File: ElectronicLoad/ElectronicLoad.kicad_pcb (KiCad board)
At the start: 4 copper layers, 101 x 64 mm, 581 parts, among them J1 AdafruitConverter, J3 Conn_01x02_Female, J4 Conn_01x02_Female, J5 Conn_01x02_Female, Q1 BUK9515-60E, Q2 BUK9515-60E, SW1 Rotary_Encoder_Switch, U1 MCP1812AT-033, U2 STM32G030C6T6, U3 MCP48CXBX1, U4 AD8605, U5 AD8605, U6 AD8605, U7 74HC595D, Y1 Crystal_GND24

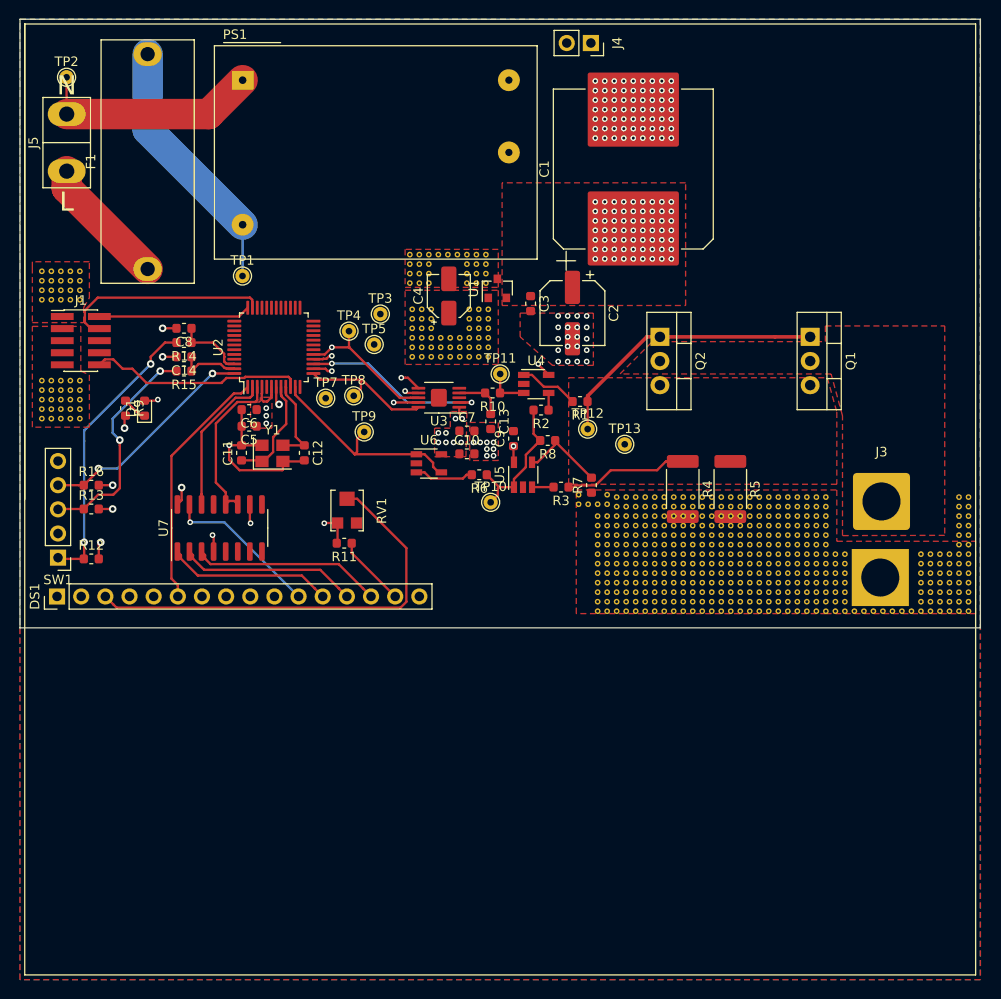
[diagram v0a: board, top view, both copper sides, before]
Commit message: Desktop
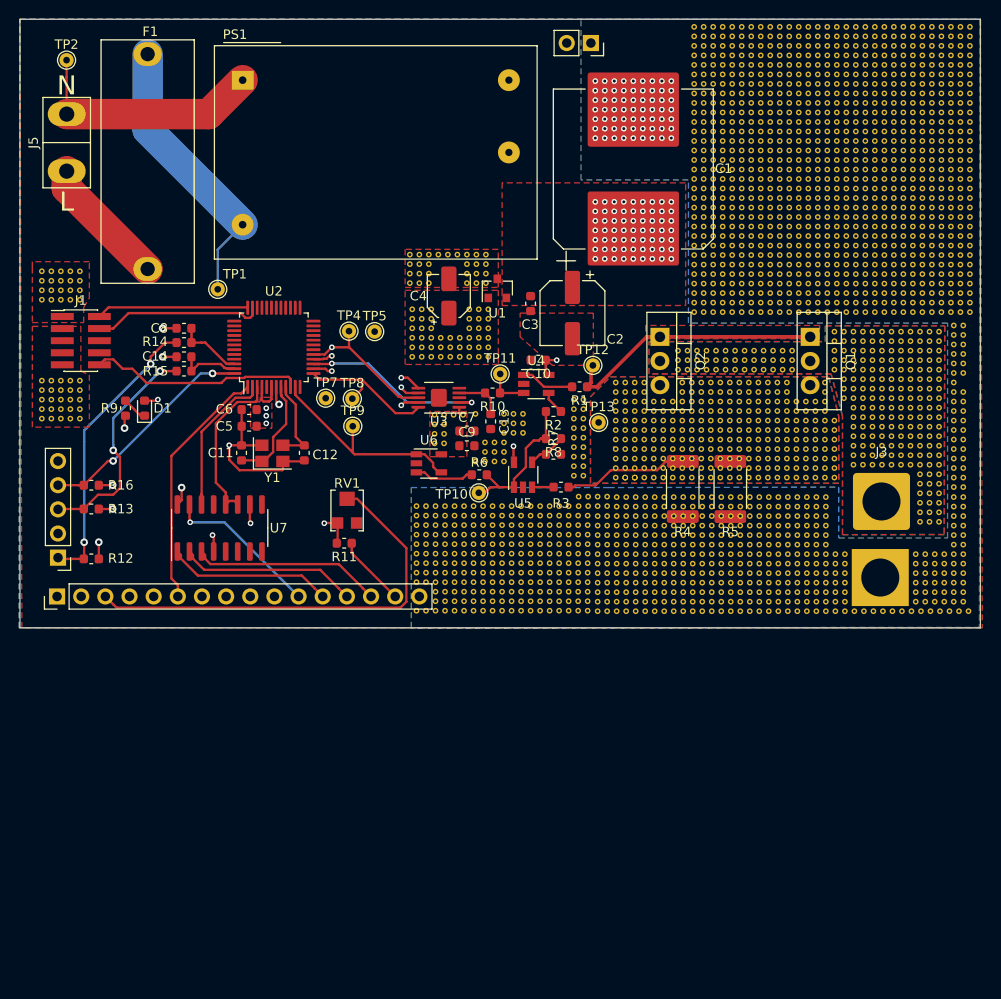
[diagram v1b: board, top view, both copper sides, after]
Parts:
- removed TP3: TestPoint, TestPoint:TestPoint_THTPad_D1.5mm_Drill0.7mm
- added REF**: VIA-0.6mm, Logan:VIA-0.6mm, F.Cu at (64.2, 92.7)
- added REF**: VIA-0.6mm, Logan:VIA-0.6mm, F.Cu at (73.8, 87.5)
- added REF**: VIA-0.6mm, Logan:VIA-0.6mm, F.Cu at (102.4, 72.3)
- added REF**: VIA-0.6mm, Logan:VIA-0.6mm, F.Cu at (102.4, 71.3)
- added REF**: VIA-0.6mm, Logan:VIA-0.6mm, F.Cu at (101.4, 71.3)
- added REF**: VIA-0.6mm, Logan:VIA-0.6mm, F.Cu at (100.4, 71.3)
- added REF**: VIA-0.6mm, Logan:VIA-0.6mm, F.Cu at (99.4, 71.3)
- added REF**: VIA-0.6mm, Logan:VIA-0.6mm, F.Cu at (98.4, 71.3)
- added REF**: VIA-0.6mm, Logan:VIA-0.6mm, F.Cu at (97.4, 71.3)
- added REF**: VIA-0.6mm, Logan:VIA-0.6mm, F.Cu at (96.4, 71.3)
- added REF**: VIA-0.6mm, Logan:VIA-0.6mm, F.Cu at (95.4, 71.3)
- added REF**: VIA-0.6mm, Logan:VIA-0.6mm, F.Cu at (94.4, 71.3)
- added REF**: VIA-0.6mm, Logan:VIA-0.6mm, F.Cu at (93.4, 71.3)
- added REF**: VIA-0.6mm, Logan:VIA-0.6mm, F.Cu at (101.4, 72.3)
- added REF**: VIA-0.6mm, Logan:VIA-0.6mm, F.Cu at (92.4, 71.3)
- added REF**: VIA-0.6mm, Logan:VIA-0.6mm, F.Cu at (91.4, 71.3)
- added REF**: VIA-0.6mm, Logan:VIA-0.6mm, F.Cu at (90.4, 71.3)
- added REF**: VIA-0.6mm, Logan:VIA-0.6mm, F.Cu at (89.4, 71.3)
- added REF**: VIA-0.6mm, Logan:VIA-0.6mm, F.Cu at (88.4, 71.3)
- added REF**: VIA-0.6mm, Logan:VIA-0.6mm, F.Cu at (87.4, 71.3)
- added REF**: VIA-0.6mm, Logan:VIA-0.6mm, F.Cu at (86.4, 71.3)
- added REF**: VIA-0.6mm, Logan:VIA-0.6mm, F.Cu at (101.2, 83.7)
- added REF**: VIA-0.6mm, Logan:VIA-0.6mm, F.Cu at (101.2, 84.7)
- added REF**: VIA-0.6mm, Logan:VIA-0.6mm, F.Cu at (101.2, 85.7)
- added REF**: VIA-0.6mm, Logan:VIA-0.6mm, F.Cu at (100.4, 72.3)
- added REF**: VIA-0.6mm, Logan:VIA-0.6mm, F.Cu at (101.2, 86.7)
- added REF**: VIA-0.6mm, Logan:VIA-0.6mm, F.Cu at (101.2, 87.7)
- added REF**: VIA-0.6mm, Logan:VIA-0.6mm, F.Cu at (101.2, 88.7)
- added REF**: VIA-0.6mm, Logan:VIA-0.6mm, F.Cu at (101.2, 89.7)
- added REF**: VIA-0.6mm, Logan:VIA-0.6mm, F.Cu at (100.2, 89.7)
- added REF**: VIA-0.6mm, Logan:VIA-0.6mm, F.Cu at (99.2, 89.7)
- added REF**: VIA-0.6mm, Logan:VIA-0.6mm, F.Cu at (98.2, 89.7)
- added REF**: VIA-0.6mm, Logan:VIA-0.6mm, F.Cu at (97.2, 89.7)
- added REF**: VIA-0.6mm, Logan:VIA-0.6mm, F.Cu at (96.2, 89.7)
- added REF**: VIA-0.6mm, Logan:VIA-0.6mm, F.Cu at (95.2, 89.7)
- added REF**: VIA-0.6mm, Logan:VIA-0.6mm, F.Cu at (99.4, 72.3)
- added REF**: VIA-0.6mm, Logan:VIA-0.6mm, F.Cu at (94.2, 89.7)
- added REF**: VIA-0.6mm, Logan:VIA-0.6mm, F.Cu at (93.2, 89.7)
- added REF**: VIA-0.6mm, Logan:VIA-0.6mm, F.Cu at (92.2, 89.7)
- added REF**: VIA-0.6mm, Logan:VIA-0.6mm, F.Cu at (91.2, 89.7)
- added REF**: VIA-0.6mm, Logan:VIA-0.6mm, F.Cu at (90.2, 89.7)
- added REF**: VIA-0.6mm, Logan:VIA-0.6mm, F.Cu at (89.2, 89.7)
- added REF**: VIA-0.6mm, Logan:VIA-0.6mm, F.Cu at (88.2, 89.7)
- added REF**: VIA-0.6mm, Logan:VIA-0.6mm, F.Cu at (87.2, 89.7)
- added REF**: VIA-0.6mm, Logan:VIA-0.6mm, F.Cu at (86.2, 89.7)
- added REF**: VIA-0.6mm, Logan:VIA-0.6mm, F.Cu at (85.2, 89.7)
- added REF**: VIA-0.6mm, Logan:VIA-0.6mm, F.Cu at (98.4, 72.3)
- added REF**: VIA-0.6mm, Logan:VIA-0.6mm, F.Cu at (84.2, 89.7)
- added REF**: VIA-0.6mm, Logan:VIA-0.6mm, F.Cu at (83.2, 89.7)
- added REF**: VIA-0.6mm, Logan:VIA-0.6mm, F.Cu at (82.2, 89.7)
- added REF**: VIA-0.6mm, Logan:VIA-0.6mm, F.Cu at (81.2, 89.7)
- added REF** (x2): VIA-0.6mm, Logan:VIA-0.6mm, F.Cu at (80.2, 89.7)
- added REF** (x2): VIA-0.6mm, Logan:VIA-0.6mm, F.Cu at (79.2, 89.7)
- added REF**: VIA-0.6mm, Logan:VIA-0.6mm, F.Cu at (100.2, 88.7)
- added REF**: VIA-0.6mm, Logan:VIA-0.6mm, F.Cu at (99.2, 88.7)
- added REF**: VIA-0.6mm, Logan:VIA-0.6mm, F.Cu at (98.2, 88.7)
- added REF**: VIA-0.6mm, Logan:VIA-0.6mm, F.Cu at (97.2, 88.7)
- added REF**: VIA-0.6mm, Logan:VIA-0.6mm, F.Cu at (97.4, 72.3)
- added REF**: VIA-0.6mm, Logan:VIA-0.6mm, F.Cu at (96.2, 88.7)
- added REF**: VIA-0.6mm, Logan:VIA-0.6mm, F.Cu at (95.2, 88.7)
- added REF**: VIA-0.6mm, Logan:VIA-0.6mm, F.Cu at (94.2, 88.7)
- added REF**: VIA-0.6mm, Logan:VIA-0.6mm, F.Cu at (93.2, 88.7)
- added REF**: VIA-0.6mm, Logan:VIA-0.6mm, F.Cu at (92.2, 88.7)
- added REF**: VIA-0.6mm, Logan:VIA-0.6mm, F.Cu at (91.2, 88.7)
- added REF**: VIA-0.6mm, Logan:VIA-0.6mm, F.Cu at (90.2, 88.7)
- added REF**: VIA-0.6mm, Logan:VIA-0.6mm, F.Cu at (89.2, 88.7)
- added REF**: VIA-0.6mm, Logan:VIA-0.6mm, F.Cu at (88.2, 88.7)
- added REF**: VIA-0.6mm, Logan:VIA-0.6mm, F.Cu at (87.2, 88.7)
- added REF**: VIA-0.6mm, Logan:VIA-0.6mm, F.Cu at (96.4, 72.3)
- added REF**: VIA-0.6mm, Logan:VIA-0.6mm, F.Cu at (86.2, 88.7)
- added REF**: VIA-0.6mm, Logan:VIA-0.6mm, F.Cu at (85.2, 88.7)
- added REF**: VIA-0.6mm, Logan:VIA-0.6mm, F.Cu at (84.2, 88.7)
- added REF**: VIA-0.6mm, Logan:VIA-0.6mm, F.Cu at (83.2, 88.7)
- added REF**: VIA-0.6mm, Logan:VIA-0.6mm, F.Cu at (82.2, 88.7)
- added REF**: VIA-0.6mm, Logan:VIA-0.6mm, F.Cu at (81.2, 88.7)
- added REF**: VIA-0.6mm, Logan:VIA-0.6mm, F.Cu at (100.2, 87.7)
- added REF**: VIA-0.6mm, Logan:VIA-0.6mm, F.Cu at (99.2, 87.7)
- added REF**: VIA-0.6mm, Logan:VIA-0.6mm, F.Cu at (98.2, 87.7)
- added REF**: VIA-0.6mm, Logan:VIA-0.6mm, F.Cu at (97.2, 87.7)
- added REF**: VIA-0.6mm, Logan:VIA-0.6mm, F.Cu at (95.4, 72.3)
- added REF**: VIA-0.6mm, Logan:VIA-0.6mm, F.Cu at (96.2, 87.7)
- added REF**: VIA-0.6mm, Logan:VIA-0.6mm, F.Cu at (95.2, 87.7)
- added REF**: VIA-0.6mm, Logan:VIA-0.6mm, F.Cu at (94.2, 87.7)
- added REF**: VIA-0.6mm, Logan:VIA-0.6mm, F.Cu at (93.2, 87.7)
- added REF**: VIA-0.6mm, Logan:VIA-0.6mm, F.Cu at (92.2, 87.7)
- added REF**: VIA-0.6mm, Logan:VIA-0.6mm, F.Cu at (91.2, 87.7)
- added REF**: VIA-0.6mm, Logan:VIA-0.6mm, F.Cu at (90.2, 87.7)
- added REF**: VIA-0.6mm, Logan:VIA-0.6mm, F.Cu at (89.2, 87.7)
- added REF**: VIA-0.6mm, Logan:VIA-0.6mm, F.Cu at (88.2, 87.7)
- added REF**: VIA-0.6mm, Logan:VIA-0.6mm, F.Cu at (87.2, 87.7)
- added REF**: VIA-0.6mm, Logan:VIA-0.6mm, F.Cu at (94.4, 72.3)
- added REF**: VIA-0.6mm, Logan:VIA-0.6mm, F.Cu at (86.2, 87.7)
- added REF**: VIA-0.6mm, Logan:VIA-0.6mm, F.Cu at (85.2, 87.7)
- added REF**: VIA-0.6mm, Logan:VIA-0.6mm, F.Cu at (84.2, 87.7)
- added REF**: VIA-0.6mm, Logan:VIA-0.6mm, F.Cu at (83.2, 87.7)
- added REF**: VIA-0.6mm, Logan:VIA-0.6mm, F.Cu at (82.2, 87.7)
- added REF**: VIA-0.6mm, Logan:VIA-0.6mm, F.Cu at (81.2, 87.7)
- added REF**: VIA-0.6mm, Logan:VIA-0.6mm, F.Cu at (100.2, 86.7)
- added REF**: VIA-0.6mm, Logan:VIA-0.6mm, F.Cu at (99.2, 86.7)
- added REF**: VIA-0.6mm, Logan:VIA-0.6mm, F.Cu at (98.2, 86.7)
- added REF**: VIA-0.6mm, Logan:VIA-0.6mm, F.Cu at (97.2, 86.7)
- added REF**: VIA-0.6mm, Logan:VIA-0.6mm, F.Cu at (93.4, 72.3)
- added REF**: VIA-0.6mm, Logan:VIA-0.6mm, F.Cu at (96.2, 86.7)
- added REF**: VIA-0.6mm, Logan:VIA-0.6mm, F.Cu at (95.2, 86.7)
- added REF**: VIA-0.6mm, Logan:VIA-0.6mm, F.Cu at (94.2, 86.7)
- added REF**: VIA-0.6mm, Logan:VIA-0.6mm, F.Cu at (93.2, 86.7)
- added REF**: VIA-0.6mm, Logan:VIA-0.6mm, F.Cu at (92.2, 86.7)
- added REF**: VIA-0.6mm, Logan:VIA-0.6mm, F.Cu at (91.2, 86.7)
- added REF**: VIA-0.6mm, Logan:VIA-0.6mm, F.Cu at (90.2, 86.7)
- added REF**: VIA-0.6mm, Logan:VIA-0.6mm, F.Cu at (89.2, 86.7)
- added REF**: VIA-0.6mm, Logan:VIA-0.6mm, F.Cu at (88.2, 86.7)
- added REF**: VIA-0.6mm, Logan:VIA-0.6mm, F.Cu at (87.2, 86.7)
- added REF**: VIA-0.6mm, Logan:VIA-0.6mm, F.Cu at (73.8, 88.5)
- added REF**: VIA-0.6mm, Logan:VIA-0.6mm, F.Cu at (92.4, 72.3)
- added REF**: VIA-0.6mm, Logan:VIA-0.6mm, F.Cu at (86.2, 86.7)
- added REF**: VIA-0.6mm, Logan:VIA-0.6mm, F.Cu at (85.2, 86.7)
- added REF**: VIA-0.6mm, Logan:VIA-0.6mm, F.Cu at (84.2, 86.7)
- added REF**: VIA-0.6mm, Logan:VIA-0.6mm, F.Cu at (83.2, 86.7)
- added REF**: VIA-0.6mm, Logan:VIA-0.6mm, F.Cu at (82.2, 86.7)
- added REF**: VIA-0.6mm, Logan:VIA-0.6mm, F.Cu at (81.2, 86.7)
- added REF**: VIA-0.6mm, Logan:VIA-0.6mm, F.Cu at (100.2, 85.7)
- added REF**: VIA-0.6mm, Logan:VIA-0.6mm, F.Cu at (99.2, 85.7)
- added REF**: VIA-0.6mm, Logan:VIA-0.6mm, F.Cu at (98.2, 85.7)
- added REF**: VIA-0.6mm, Logan:VIA-0.6mm, F.Cu at (97.2, 85.7)
- added REF**: VIA-0.6mm, Logan:VIA-0.6mm, F.Cu at (91.4, 72.3)
- added REF**: VIA-0.6mm, Logan:VIA-0.6mm, F.Cu at (96.2, 85.7)
- added REF**: VIA-0.6mm, Logan:VIA-0.6mm, F.Cu at (95.2, 85.7)
- added REF**: VIA-0.6mm, Logan:VIA-0.6mm, F.Cu at (94.2, 85.7)
- added REF**: VIA-0.6mm, Logan:VIA-0.6mm, F.Cu at (93.2, 85.7)
- added REF**: VIA-0.6mm, Logan:VIA-0.6mm, F.Cu at (92.2, 85.7)
- added REF**: VIA-0.6mm, Logan:VIA-0.6mm, F.Cu at (91.2, 85.7)
- added REF**: VIA-0.6mm, Logan:VIA-0.6mm, F.Cu at (90.2, 85.7)
- added REF**: VIA-0.6mm, Logan:VIA-0.6mm, F.Cu at (89.2, 85.7)
- added REF**: VIA-0.6mm, Logan:VIA-0.6mm, F.Cu at (88.2, 85.7)
- added REF**: VIA-0.6mm, Logan:VIA-0.6mm, F.Cu at (87.2, 85.7)
- added REF**: VIA-0.6mm, Logan:VIA-0.6mm, F.Cu at (90.4, 72.3)
- added REF**: VIA-0.6mm, Logan:VIA-0.6mm, F.Cu at (86.2, 85.7)
- added REF**: VIA-0.6mm, Logan:VIA-0.6mm, F.Cu at (85.2, 85.7)
- added REF**: VIA-0.6mm, Logan:VIA-0.6mm, F.Cu at (84.2, 85.7)
- added REF**: VIA-0.6mm, Logan:VIA-0.6mm, F.Cu at (83.2, 85.7)
- added REF**: VIA-0.6mm, Logan:VIA-0.6mm, F.Cu at (82.2, 85.7)
- added REF**: VIA-0.6mm, Logan:VIA-0.6mm, F.Cu at (81.2, 85.7)
- added REF**: VIA-0.6mm, Logan:VIA-0.6mm, F.Cu at (100.2, 84.7)
- added REF**: VIA-0.6mm, Logan:VIA-0.6mm, F.Cu at (99.2, 84.7)
- added REF**: VIA-0.6mm, Logan:VIA-0.6mm, F.Cu at (98.2, 84.7)
- added REF**: VIA-0.6mm, Logan:VIA-0.6mm, F.Cu at (97.2, 84.7)
- added REF**: VIA-0.6mm, Logan:VIA-0.6mm, F.Cu at (89.4, 72.3)
- added REF**: VIA-0.6mm, Logan:VIA-0.6mm, F.Cu at (96.2, 84.7)
- added REF**: VIA-0.6mm, Logan:VIA-0.6mm, F.Cu at (95.2, 84.7)
- added REF**: VIA-0.6mm, Logan:VIA-0.6mm, F.Cu at (94.2, 84.7)
- added REF**: VIA-0.6mm, Logan:VIA-0.6mm, F.Cu at (93.2, 84.7)
- added REF**: VIA-0.6mm, Logan:VIA-0.6mm, F.Cu at (92.2, 84.7)
- added REF**: VIA-0.6mm, Logan:VIA-0.6mm, F.Cu at (91.2, 84.7)
- added REF**: VIA-0.6mm, Logan:VIA-0.6mm, F.Cu at (90.2, 84.7)
- added REF**: VIA-0.6mm, Logan:VIA-0.6mm, F.Cu at (89.2, 84.7)
- added REF**: VIA-0.6mm, Logan:VIA-0.6mm, F.Cu at (88.2, 84.7)
- added REF**: VIA-0.6mm, Logan:VIA-0.6mm, F.Cu at (87.2, 84.7)
- added REF**: VIA-0.6mm, Logan:VIA-0.6mm, F.Cu at (88.4, 72.3)
- added REF**: VIA-0.6mm, Logan:VIA-0.6mm, F.Cu at (86.2, 84.7)
- added REF**: VIA-0.6mm, Logan:VIA-0.6mm, F.Cu at (85.2, 84.7)
- added REF**: VIA-0.6mm, Logan:VIA-0.6mm, F.Cu at (84.2, 84.7)
- added REF**: VIA-0.6mm, Logan:VIA-0.6mm, F.Cu at (83.2, 84.7)
- added REF**: VIA-0.6mm, Logan:VIA-0.6mm, F.Cu at (82.2, 84.7)
- added REF**: VIA-0.6mm, Logan:VIA-0.6mm, F.Cu at (81.2, 84.7)
- added REF**: VIA-0.6mm, Logan:VIA-0.6mm, F.Cu at (78.2, 79.7)
- added REF**: VIA-0.6mm, Logan:VIA-0.6mm, F.Cu at (79.2, 79.7)
- added REF**: VIA-0.6mm, Logan:VIA-0.6mm, F.Cu at (80.2, 79.7)
- added REF**: VIA-0.6mm, Logan:VIA-0.6mm, F.Cu at (100.2, 83.7)
- added REF**: VIA-0.6mm, Logan:VIA-0.6mm, F.Cu at (87.4, 72.3)
- added REF**: VIA-0.6mm, Logan:VIA-0.6mm, F.Cu at (99.2, 83.7)
- added REF**: VIA-0.6mm, Logan:VIA-0.6mm, F.Cu at (98.2, 83.7)
- added REF**: VIA-0.6mm, Logan:VIA-0.6mm, F.Cu at (97.2, 83.7)
- added REF**: VIA-0.6mm, Logan:VIA-0.6mm, F.Cu at (96.2, 83.7)
- added REF**: VIA-0.6mm, Logan:VIA-0.6mm, F.Cu at (95.2, 83.7)
- added REF**: VIA-0.6mm, Logan:VIA-0.6mm, F.Cu at (94.2, 83.7)
- added REF**: VIA-0.6mm, Logan:VIA-0.6mm, F.Cu at (93.2, 83.7)
- added REF**: VIA-0.6mm, Logan:VIA-0.6mm, F.Cu at (92.2, 83.7)
- added REF**: VIA-0.6mm, Logan:VIA-0.6mm, F.Cu at (91.2, 83.7)
- added REF**: VIA-0.6mm, Logan:VIA-0.6mm, F.Cu at (90.2, 83.7)
- added REF**: VIA-0.6mm, Logan:VIA-0.6mm, F.Cu at (86.4, 72.3)
- added REF**: VIA-0.6mm, Logan:VIA-0.6mm, F.Cu at (89.2, 83.7)
- added REF**: VIA-0.6mm, Logan:VIA-0.6mm, F.Cu at (88.2, 83.7)
- added REF**: VIA-0.6mm, Logan:VIA-0.6mm, F.Cu at (87.2, 83.7)
- added REF**: VIA-0.6mm, Logan:VIA-0.6mm, F.Cu at (86.2, 83.7)
- added REF**: VIA-0.6mm, Logan:VIA-0.6mm, F.Cu at (85.2, 83.7)
- added REF**: VIA-0.6mm, Logan:VIA-0.6mm, F.Cu at (84.2, 83.7)
- added REF**: VIA-0.6mm, Logan:VIA-0.6mm, F.Cu at (83.2, 83.7)
- added REF**: VIA-0.6mm, Logan:VIA-0.6mm, F.Cu at (82.2, 83.7)
- added REF**: VIA-0.6mm, Logan:VIA-0.6mm, F.Cu at (81.2, 83.7)
- added REF**: VIA-0.6mm, Logan:VIA-0.6mm, F.Cu at (78.2, 80.7)
- added REF**: VIA-0.6mm, Logan:VIA-0.6mm, F.Cu at (115.4, 42.3)
- added REF**: VIA-0.6mm, Logan:VIA-0.6mm, F.Cu at (79.2, 80.7)
- added REF**: VIA-0.6mm, Logan:VIA-0.6mm, F.Cu at (80.2, 80.7)
- added REF**: VIA-0.6mm, Logan:VIA-0.6mm, F.Cu at (100.2, 82.7)
- added REF**: VIA-0.6mm, Logan:VIA-0.6mm, F.Cu at (99.2, 82.7)
- added REF**: VIA-0.6mm, Logan:VIA-0.6mm, F.Cu at (98.2, 82.7)
- added REF**: VIA-0.6mm, Logan:VIA-0.6mm, F.Cu at (97.2, 82.7)
- added REF**: VIA-0.6mm, Logan:VIA-0.6mm, F.Cu at (96.2, 82.7)
- added REF**: VIA-0.6mm, Logan:VIA-0.6mm, F.Cu at (95.2, 82.7)
- added REF**: VIA-0.6mm, Logan:VIA-0.6mm, F.Cu at (94.2, 82.7)
- added REF**: VIA-0.6mm, Logan:VIA-0.6mm, F.Cu at (93.2, 82.7)
- added REF**: VIA-0.6mm, Logan:VIA-0.6mm, F.Cu at (114.4, 42.3)
- added REF**: VIA-0.6mm, Logan:VIA-0.6mm, F.Cu at (92.2, 82.7)
- added REF**: VIA-0.6mm, Logan:VIA-0.6mm, F.Cu at (91.2, 82.7)
- added REF**: VIA-0.6mm, Logan:VIA-0.6mm, F.Cu at (90.2, 82.7)
- added REF**: VIA-0.6mm, Logan:VIA-0.6mm, F.Cu at (89.2, 82.7)
- added REF**: VIA-0.6mm, Logan:VIA-0.6mm, F.Cu at (88.2, 82.7)
- added REF**: VIA-0.6mm, Logan:VIA-0.6mm, F.Cu at (87.2, 82.7)
- added REF**: VIA-0.6mm, Logan:VIA-0.6mm, F.Cu at (86.2, 82.7)
- added REF**: VIA-0.6mm, Logan:VIA-0.6mm, F.Cu at (85.2, 82.7)
- added REF**: VIA-0.6mm, Logan:VIA-0.6mm, F.Cu at (84.2, 82.7)
- added REF**: VIA-0.6mm, Logan:VIA-0.6mm, F.Cu at (83.2, 82.7)
- added REF**: VIA-0.6mm, Logan:VIA-0.6mm, F.Cu at (113.4, 42.3)
- added REF**: VIA-0.6mm, Logan:VIA-0.6mm, F.Cu at (82.2, 82.7)
- added REF**: VIA-0.6mm, Logan:VIA-0.6mm, F.Cu at (81.2, 82.7)
- added REF**: VIA-0.6mm, Logan:VIA-0.6mm, F.Cu at (78.2, 81.7)
- added REF**: VIA-0.6mm, Logan:VIA-0.6mm, F.Cu at (79.2, 81.7)
- added REF**: VIA-0.6mm, Logan:VIA-0.6mm, F.Cu at (80.2, 81.7)
- added REF**: VIA-0.6mm, Logan:VIA-0.6mm, F.Cu at (100.2, 81.7)
- added REF**: VIA-0.6mm, Logan:VIA-0.6mm, F.Cu at (99.2, 81.7)
- added REF**: VIA-0.6mm, Logan:VIA-0.6mm, F.Cu at (98.2, 81.7)
- added REF**: VIA-0.6mm, Logan:VIA-0.6mm, F.Cu at (97.2, 81.7)
- added REF**: VIA-0.6mm, Logan:VIA-0.6mm, F.Cu at (96.2, 81.7)
- added REF**: VIA-0.6mm, Logan:VIA-0.6mm, F.Cu at (73.8, 89.5)
- added REF**: VIA-0.6mm, Logan:VIA-0.6mm, F.Cu at (112.4, 42.3)
- added REF**: VIA-0.6mm, Logan:VIA-0.6mm, F.Cu at (95.2, 81.7)
- added REF**: VIA-0.6mm, Logan:VIA-0.6mm, F.Cu at (94.2, 81.7)
- added REF**: VIA-0.6mm, Logan:VIA-0.6mm, F.Cu at (93.2, 81.7)
- added REF**: VIA-0.6mm, Logan:VIA-0.6mm, F.Cu at (92.2, 81.7)
- added REF**: VIA-0.6mm, Logan:VIA-0.6mm, F.Cu at (91.2, 81.7)
- added REF**: VIA-0.6mm, Logan:VIA-0.6mm, F.Cu at (90.2, 81.7)
- added REF**: VIA-0.6mm, Logan:VIA-0.6mm, F.Cu at (89.2, 81.7)
- added REF**: VIA-0.6mm, Logan:VIA-0.6mm, F.Cu at (88.2, 81.7)
- added REF**: VIA-0.6mm, Logan:VIA-0.6mm, F.Cu at (87.2, 81.7)
- added REF**: VIA-0.6mm, Logan:VIA-0.6mm, F.Cu at (86.2, 81.7)
- added REF**: VIA-0.6mm, Logan:VIA-0.6mm, F.Cu at (111.4, 42.3)
- added REF**: VIA-0.6mm, Logan:VIA-0.6mm, F.Cu at (85.2, 81.7)
- added REF**: VIA-0.6mm, Logan:VIA-0.6mm, F.Cu at (84.2, 81.7)
- added REF**: VIA-0.6mm, Logan:VIA-0.6mm, F.Cu at (83.2, 81.7)
- added REF**: VIA-0.6mm, Logan:VIA-0.6mm, F.Cu at (82.2, 81.7)
- added REF**: VIA-0.6mm, Logan:VIA-0.6mm, F.Cu at (81.2, 81.7)
- added REF**: VIA-0.6mm, Logan:VIA-0.6mm, F.Cu at (78.2, 82.7)
- added REF**: VIA-0.6mm, Logan:VIA-0.6mm, F.Cu at (79.2, 82.7)
- added REF**: VIA-0.6mm, Logan:VIA-0.6mm, F.Cu at (80.2, 82.7)
- added REF**: VIA-0.6mm, Logan:VIA-0.6mm, F.Cu at (100.2, 80.7)
- added REF**: VIA-0.6mm, Logan:VIA-0.6mm, F.Cu at (96.2, 80.7)
- added REF**: VIA-0.6mm, Logan:VIA-0.6mm, F.Cu at (110.4, 42.3)
- added REF**: VIA-0.6mm, Logan:VIA-0.6mm, F.Cu at (95.2, 80.7)
- added REF**: VIA-0.6mm, Logan:VIA-0.6mm, F.Cu at (94.2, 80.7)
- added REF**: VIA-0.6mm, Logan:VIA-0.6mm, F.Cu at (93.2, 80.7)
- added REF**: VIA-0.6mm, Logan:VIA-0.6mm, F.Cu at (92.2, 80.7)
- added REF**: VIA-0.6mm, Logan:VIA-0.6mm, F.Cu at (91.2, 80.7)
- added REF**: VIA-0.6mm, Logan:VIA-0.6mm, F.Cu at (90.2, 80.7)
- added REF**: VIA-0.6mm, Logan:VIA-0.6mm, F.Cu at (89.2, 80.7)
- added REF**: VIA-0.6mm, Logan:VIA-0.6mm, F.Cu at (88.2, 80.7)
- added REF**: VIA-0.6mm, Logan:VIA-0.6mm, F.Cu at (87.2, 80.7)
- added REF**: VIA-0.6mm, Logan:VIA-0.6mm, F.Cu at (86.2, 80.7)
- added REF**: VIA-0.6mm, Logan:VIA-0.6mm, F.Cu at (109.4, 42.3)
- added REF**: VIA-0.6mm, Logan:VIA-0.6mm, F.Cu at (85.2, 80.7)
- added REF**: VIA-0.6mm, Logan:VIA-0.6mm, F.Cu at (81.2, 80.7)
- added REF**: VIA-0.6mm, Logan:VIA-0.6mm, F.Cu at (78.2, 83.7)
- added REF**: VIA-0.6mm, Logan:VIA-0.6mm, F.Cu at (79.2, 83.7)
- added REF**: VIA-0.6mm, Logan:VIA-0.6mm, F.Cu at (80.2, 83.7)
- added REF**: VIA-0.6mm, Logan:VIA-0.6mm, F.Cu at (100.2, 79.7)
- added REF**: VIA-0.6mm, Logan:VIA-0.6mm, F.Cu at (96.2, 79.7)
- added REF**: VIA-0.6mm, Logan:VIA-0.6mm, F.Cu at (95.2, 79.7)
- added REF**: VIA-0.6mm, Logan:VIA-0.6mm, F.Cu at (94.2, 79.7)
- added REF**: VIA-0.6mm, Logan:VIA-0.6mm, F.Cu at (93.2, 79.7)
- added REF**: VIA-0.6mm, Logan:VIA-0.6mm, F.Cu at (108.4, 42.3)
- added REF**: VIA-0.6mm, Logan:VIA-0.6mm, F.Cu at (92.2, 79.7)
- added REF**: VIA-0.6mm, Logan:VIA-0.6mm, F.Cu at (91.2, 79.7)
- added REF**: VIA-0.6mm, Logan:VIA-0.6mm, F.Cu at (90.2, 79.7)
- added REF**: VIA-0.6mm, Logan:VIA-0.6mm, F.Cu at (89.2, 79.7)
- added REF**: VIA-0.6mm, Logan:VIA-0.6mm, F.Cu at (88.2, 79.7)
- added REF**: VIA-0.6mm, Logan:VIA-0.6mm, F.Cu at (87.2, 79.7)
- added REF**: VIA-0.6mm, Logan:VIA-0.6mm, F.Cu at (86.2, 79.7)
- added REF**: VIA-0.6mm, Logan:VIA-0.6mm, F.Cu at (85.2, 79.7)
- added REF**: VIA-0.6mm, Logan:VIA-0.6mm, F.Cu at (81.2, 79.7)
- added REF**: VIA-0.6mm, Logan:VIA-0.6mm, F.Cu at (78.2, 84.7)
- added REF**: VIA-0.6mm, Logan:VIA-0.6mm, F.Cu at (107.4, 42.3)
- added REF**: VIA-0.6mm, Logan:VIA-0.6mm, F.Cu at (79.2, 84.7)
- added REF**: VIA-0.6mm, Logan:VIA-0.6mm, F.Cu at (80.2, 84.7)
- added REF**: VIA-0.6mm, Logan:VIA-0.6mm, F.Cu at (78.2, 85.7)
- added REF**: VIA-0.6mm, Logan:VIA-0.6mm, F.Cu at (79.2, 85.7)
- added REF**: VIA-0.6mm, Logan:VIA-0.6mm, F.Cu at (80.2, 85.7)
- added REF**: VIA-0.6mm, Logan:VIA-0.6mm, F.Cu at (78.2, 86.7)
- added REF**: VIA-0.6mm, Logan:VIA-0.6mm, F.Cu at (79.2, 86.7)
- added REF**: VIA-0.6mm, Logan:VIA-0.6mm, F.Cu at (80.2, 86.7)
- added REF**: VIA-0.6mm, Logan:VIA-0.6mm, F.Cu at (78.2, 87.7)
- added REF**: VIA-0.6mm, Logan:VIA-0.6mm, F.Cu at (79.2, 87.7)
- added REF**: VIA-0.6mm, Logan:VIA-0.6mm, F.Cu at (106.4, 42.3)
- added REF**: VIA-0.6mm, Logan:VIA-0.6mm, F.Cu at (80.2, 87.7)
- added REF**: VIA-0.6mm, Logan:VIA-0.6mm, F.Cu at (78.2, 88.7)
- added REF**: VIA-0.6mm, Logan:VIA-0.6mm, F.Cu at (79.2, 88.7)
- added REF**: VIA-0.6mm, Logan:VIA-0.6mm, F.Cu at (80.2, 88.7)
- added REF**: VIA-0.6mm, Logan:VIA-0.6mm, F.Cu at (78.2, 89.7)
- added REF**: VIA-0.6mm, Logan:VIA-0.6mm, F.Cu at (110.2, 93.3)
- added REF**: VIA-0.6mm, Logan:VIA-0.6mm, F.Cu at (111.2, 93.3)
- added REF**: VIA-0.6mm, Logan:VIA-0.6mm, F.Cu at (112.2, 93.3)
- added REF**: VIA-0.6mm, Logan:VIA-0.6mm, F.Cu at (105.4, 42.3)
- added REF**: VIA-0.6mm, Logan:VIA-0.6mm, F.Cu at (110.2, 94.3)
- added REF**: VIA-0.6mm, Logan:VIA-0.6mm, F.Cu at (111.2, 94.3)
- added REF**: VIA-0.6mm, Logan:VIA-0.6mm, F.Cu at (112.2, 94.3)
- added REF**: VIA-0.6mm, Logan:VIA-0.6mm, F.Cu at (110.2, 92.3)
- added REF**: VIA-0.6mm, Logan:VIA-0.6mm, F.Cu at (111.2, 92.3)
- added REF**: VIA-0.6mm, Logan:VIA-0.6mm, F.Cu at (112.2, 92.3)
- added REF**: VIA-0.6mm, Logan:VIA-0.6mm, F.Cu at (103.2, 88.3)
- added REF**: VIA-0.6mm, Logan:VIA-0.6mm, F.Cu at (101.2, 78.3)
- added REF**: VIA-0.6mm, Logan:VIA-0.6mm, F.Cu at (110.2, 91.3)
- added REF**: VIA-0.6mm, Logan:VIA-0.6mm, F.Cu at (111.2, 91.3)
- added REF**: VIA-0.6mm, Logan:VIA-0.6mm, F.Cu at (104.4, 42.3)
- added REF**: VIA-0.6mm, Logan:VIA-0.6mm, F.Cu at (112.2, 91.3)
- added REF**: VIA-0.6mm, Logan:VIA-0.6mm, F.Cu at (101.2, 77.3)
- added REF**: VIA-0.6mm, Logan:VIA-0.6mm, F.Cu at (110.2, 90.3)
- added REF**: VIA-0.6mm, Logan:VIA-0.6mm, F.Cu at (111.2, 90.3)
- added REF**: VIA-0.6mm, Logan:VIA-0.6mm, F.Cu at (112.2, 90.3)
- added REF**: VIA-0.6mm, Logan:VIA-0.6mm, F.Cu at (101.2, 76.3)
- added REF**: VIA-0.6mm, Logan:VIA-0.6mm, F.Cu at (110.2, 89.3)
- added REF**: VIA-0.6mm, Logan:VIA-0.6mm, F.Cu at (111.2, 89.3)
- added REF**: VIA-0.6mm, Logan:VIA-0.6mm, F.Cu at (112.2, 89.3)
- added REF**: VIA-0.6mm, Logan:VIA-0.6mm, F.Cu at (101.2, 75.3)
- added REF**: VIA-0.6mm, Logan:VIA-0.6mm, F.Cu at (103.4, 42.3)
- added REF**: VIA-0.6mm, Logan:VIA-0.6mm, F.Cu at (104.2, 88.3)
- added REF**: VIA-0.6mm, Logan:VIA-0.6mm, F.Cu at (105.2, 88.3)
- added REF**: VIA-0.6mm, Logan:VIA-0.6mm, F.Cu at (106.2, 88.3)
- added REF**: VIA-0.6mm, Logan:VIA-0.6mm, F.Cu at (107.2, 88.3)
- added REF**: VIA-0.6mm, Logan:VIA-0.6mm, F.Cu at (108.2, 88.3)
- added REF**: VIA-0.6mm, Logan:VIA-0.6mm, F.Cu at (109.2, 88.3)
- added REF**: VIA-0.6mm, Logan:VIA-0.6mm, F.Cu at (110.2, 88.3)
- added REF**: VIA-0.6mm, Logan:VIA-0.6mm, F.Cu at (111.2, 88.3)
- added REF**: VIA-0.6mm, Logan:VIA-0.6mm, F.Cu at (112.2, 88.3)
- added REF**: VIA-0.6mm, Logan:VIA-0.6mm, F.Cu at (101.2, 74.3)
- added REF**: VIA-0.6mm, Logan:VIA-0.6mm, F.Cu at (74.8, 81.5)
- added REF**: VIA-0.6mm, Logan:VIA-0.6mm, F.Cu at (102.4, 42.3)
- added REF**: VIA-0.6mm, Logan:VIA-0.6mm, F.Cu at (104.2, 87.3)
- added REF**: VIA-0.6mm, Logan:VIA-0.6mm, F.Cu at (105.2, 87.3)
- added REF**: VIA-0.6mm, Logan:VIA-0.6mm, F.Cu at (106.2, 87.3)
- added REF**: VIA-0.6mm, Logan:VIA-0.6mm, F.Cu at (107.2, 87.3)
- added REF**: VIA-0.6mm, Logan:VIA-0.6mm, F.Cu at (108.2, 87.3)
- added REF**: VIA-0.6mm, Logan:VIA-0.6mm, F.Cu at (109.2, 87.3)
- added REF**: VIA-0.6mm, Logan:VIA-0.6mm, F.Cu at (110.2, 87.3)
- added REF**: VIA-0.6mm, Logan:VIA-0.6mm, F.Cu at (111.2, 87.3)
- added REF**: VIA-0.6mm, Logan:VIA-0.6mm, F.Cu at (112.2, 87.3)
- added REF**: VIA-0.6mm, Logan:VIA-0.6mm, F.Cu at (103.2, 87.3)
- added REF**: VIA-0.6mm, Logan:VIA-0.6mm, F.Cu at (101.4, 42.3)
- added REF**: VIA-0.6mm, Logan:VIA-0.6mm, F.Cu at (104.2, 86.3)
- added REF**: VIA-0.6mm, Logan:VIA-0.6mm, F.Cu at (105.2, 86.3)
- added REF**: VIA-0.6mm, Logan:VIA-0.6mm, F.Cu at (106.2, 86.3)
- added REF**: VIA-0.6mm, Logan:VIA-0.6mm, F.Cu at (107.2, 86.3)
- added REF**: VIA-0.6mm, Logan:VIA-0.6mm, F.Cu at (108.2, 86.3)
- added REF**: VIA-0.6mm, Logan:VIA-0.6mm, F.Cu at (109.2, 86.3)
- added REF**: VIA-0.6mm, Logan:VIA-0.6mm, F.Cu at (110.2, 86.3)
- added REF**: VIA-0.6mm, Logan:VIA-0.6mm, F.Cu at (111.2, 86.3)
- added REF**: VIA-0.6mm, Logan:VIA-0.6mm, F.Cu at (112.2, 86.3)
- added REF**: VIA-0.6mm, Logan:VIA-0.6mm, F.Cu at (103.2, 86.3)
- added REF**: VIA-0.6mm, Logan:VIA-0.6mm, F.Cu at (100.4, 42.3)
- added REF**: VIA-0.6mm, Logan:VIA-0.6mm, F.Cu at (104.2, 85.3)
- added REF**: VIA-0.6mm, Logan:VIA-0.6mm, F.Cu at (105.2, 85.3)
- added REF**: VIA-0.6mm, Logan:VIA-0.6mm, F.Cu at (106.2, 85.3)
- added REF**: VIA-0.6mm, Logan:VIA-0.6mm, F.Cu at (107.2, 85.3)
- added REF**: VIA-0.6mm, Logan:VIA-0.6mm, F.Cu at (108.2, 85.3)
- added REF**: VIA-0.6mm, Logan:VIA-0.6mm, F.Cu at (109.2, 85.3)
- added REF**: VIA-0.6mm, Logan:VIA-0.6mm, F.Cu at (110.2, 85.3)
- added REF**: VIA-0.6mm, Logan:VIA-0.6mm, F.Cu at (111.2, 85.3)
- added REF**: VIA-0.6mm, Logan:VIA-0.6mm, F.Cu at (112.2, 85.3)
- added REF**: VIA-0.6mm, Logan:VIA-0.6mm, F.Cu at (103.2, 85.3)
- added REF**: VIA-0.6mm, Logan:VIA-0.6mm, F.Cu at (99.4, 42.3)
- added REF**: VIA-0.6mm, Logan:VIA-0.6mm, F.Cu at (104.2, 84.3)
- added REF**: VIA-0.6mm, Logan:VIA-0.6mm, F.Cu at (105.2, 84.3)
- added REF**: VIA-0.6mm, Logan:VIA-0.6mm, F.Cu at (106.2, 84.3)
- added REF**: VIA-0.6mm, Logan:VIA-0.6mm, F.Cu at (107.2, 84.3)
- added REF**: VIA-0.6mm, Logan:VIA-0.6mm, F.Cu at (108.2, 84.3)
- added REF**: VIA-0.6mm, Logan:VIA-0.6mm, F.Cu at (109.2, 84.3)
- added REF**: VIA-0.6mm, Logan:VIA-0.6mm, F.Cu at (110.2, 84.3)
- added REF**: VIA-0.6mm, Logan:VIA-0.6mm, F.Cu at (111.2, 84.3)
- added REF**: VIA-0.6mm, Logan:VIA-0.6mm, F.Cu at (112.2, 84.3)
- added REF**: VIA-0.6mm, Logan:VIA-0.6mm, F.Cu at (103.2, 84.3)
- added REF**: VIA-0.6mm, Logan:VIA-0.6mm, F.Cu at (98.4, 42.3)
- added REF**: VIA-0.6mm, Logan:VIA-0.6mm, F.Cu at (104.2, 83.3)
- added REF**: VIA-0.6mm, Logan:VIA-0.6mm, F.Cu at (105.2, 83.3)
- added REF**: VIA-0.6mm, Logan:VIA-0.6mm, F.Cu at (106.2, 83.3)
- added REF**: VIA-0.6mm, Logan:VIA-0.6mm, F.Cu at (107.2, 83.3)
- added REF**: VIA-0.6mm, Logan:VIA-0.6mm, F.Cu at (108.2, 83.3)
- added REF**: VIA-0.6mm, Logan:VIA-0.6mm, F.Cu at (109.2, 83.3)
- added REF**: VIA-0.6mm, Logan:VIA-0.6mm, F.Cu at (110.2, 83.3)
- added REF**: VIA-0.6mm, Logan:VIA-0.6mm, F.Cu at (111.2, 83.3)
- added REF**: VIA-0.6mm, Logan:VIA-0.6mm, F.Cu at (112.2, 83.3)
- added REF**: VIA-0.6mm, Logan:VIA-0.6mm, F.Cu at (103.2, 83.3)
- added REF**: VIA-0.6mm, Logan:VIA-0.6mm, F.Cu at (97.4, 42.3)
- added REF**: VIA-0.6mm, Logan:VIA-0.6mm, F.Cu at (104.2, 82.3)
- added REF**: VIA-0.6mm, Logan:VIA-0.6mm, F.Cu at (105.2, 82.3)
- added REF**: VIA-0.6mm, Logan:VIA-0.6mm, F.Cu at (106.2, 82.3)
- added REF**: VIA-0.6mm, Logan:VIA-0.6mm, F.Cu at (107.2, 82.3)
- added REF**: VIA-0.6mm, Logan:VIA-0.6mm, F.Cu at (108.2, 82.3)
- added REF**: VIA-0.6mm, Logan:VIA-0.6mm, F.Cu at (109.2, 82.3)
- added REF**: VIA-0.6mm, Logan:VIA-0.6mm, F.Cu at (110.2, 82.3)
- added REF**: VIA-0.6mm, Logan:VIA-0.6mm, F.Cu at (111.2, 82.3)
- added REF**: VIA-0.6mm, Logan:VIA-0.6mm, F.Cu at (112.2, 82.3)
- added REF**: VIA-0.6mm, Logan:VIA-0.6mm, F.Cu at (103.2, 82.3)
- added REF**: VIA-0.6mm, Logan:VIA-0.6mm, F.Cu at (96.4, 42.3)
- added REF**: VIA-0.6mm, Logan:VIA-0.6mm, F.Cu at (104.2, 81.3)
- added REF**: VIA-0.6mm, Logan:VIA-0.6mm, F.Cu at (105.2, 81.3)
- added REF**: VIA-0.6mm, Logan:VIA-0.6mm, F.Cu at (106.2, 81.3)
- added REF**: VIA-0.6mm, Logan:VIA-0.6mm, F.Cu at (107.2, 81.3)
- added REF**: VIA-0.6mm, Logan:VIA-0.6mm, F.Cu at (108.2, 81.3)
- added REF**: VIA-0.6mm, Logan:VIA-0.6mm, F.Cu at (109.2, 81.3)
- added REF**: VIA-0.6mm, Logan:VIA-0.6mm, F.Cu at (110.2, 81.3)
- added REF**: VIA-0.6mm, Logan:VIA-0.6mm, F.Cu at (111.2, 81.3)
- added REF**: VIA-0.6mm, Logan:VIA-0.6mm, F.Cu at (112.2, 81.3)
- added REF**: VIA-0.6mm, Logan:VIA-0.6mm, F.Cu at (102.2, 81.3)
- added REF**: VIA-0.6mm, Logan:VIA-0.6mm, F.Cu at (95.4, 42.3)
- added REF**: VIA-0.6mm, Logan:VIA-0.6mm, F.Cu at (103.2, 81.3)
- added REF**: VIA-0.6mm, Logan:VIA-0.6mm, F.Cu at (104.2, 80.3)
- added REF**: VIA-0.6mm, Logan:VIA-0.6mm, F.Cu at (105.2, 80.3)
- added REF**: VIA-0.6mm, Logan:VIA-0.6mm, F.Cu at (106.2, 80.3)
- added REF**: VIA-0.6mm, Logan:VIA-0.6mm, F.Cu at (107.2, 80.3)
- added REF**: VIA-0.6mm, Logan:VIA-0.6mm, F.Cu at (108.2, 80.3)
- added REF**: VIA-0.6mm, Logan:VIA-0.6mm, F.Cu at (109.2, 80.3)
- added REF**: VIA-0.6mm, Logan:VIA-0.6mm, F.Cu at (110.2, 80.3)
- added REF**: VIA-0.6mm, Logan:VIA-0.6mm, F.Cu at (111.2, 80.3)
- added REF**: VIA-0.6mm, Logan:VIA-0.6mm, F.Cu at (112.2, 80.3)
- added REF**: VIA-0.6mm, Logan:VIA-0.6mm, F.Cu at (94.4, 42.3)
- added REF**: VIA-0.6mm, Logan:VIA-0.6mm, F.Cu at (102.2, 80.3)
- added REF**: VIA-0.6mm, Logan:VIA-0.6mm, F.Cu at (103.2, 80.3)
- added REF**: VIA-0.6mm, Logan:VIA-0.6mm, F.Cu at (104.2, 79.3)
- added REF**: VIA-0.6mm, Logan:VIA-0.6mm, F.Cu at (105.2, 79.3)
- added REF**: VIA-0.6mm, Logan:VIA-0.6mm, F.Cu at (106.2, 79.3)
- added REF**: VIA-0.6mm, Logan:VIA-0.6mm, F.Cu at (107.2, 79.3)
- added REF**: VIA-0.6mm, Logan:VIA-0.6mm, F.Cu at (108.2, 79.3)
- added REF**: VIA-0.6mm, Logan:VIA-0.6mm, F.Cu at (109.2, 79.3)
- added REF**: VIA-0.6mm, Logan:VIA-0.6mm, F.Cu at (110.2, 79.3)
- added REF**: VIA-0.6mm, Logan:VIA-0.6mm, F.Cu at (111.2, 79.3)
- added REF**: VIA-0.6mm, Logan:VIA-0.6mm, F.Cu at (93.4, 42.3)
- added REF**: VIA-0.6mm, Logan:VIA-0.6mm, F.Cu at (112.2, 79.3)
- added REF**: VIA-0.6mm, Logan:VIA-0.6mm, F.Cu at (102.2, 79.3)
- added REF**: VIA-0.6mm, Logan:VIA-0.6mm, F.Cu at (103.2, 79.3)
- added REF**: VIA-0.6mm, Logan:VIA-0.6mm, F.Cu at (104.2, 78.3)
- added REF**: VIA-0.6mm, Logan:VIA-0.6mm, F.Cu at (105.2, 78.3)
- added REF**: VIA-0.6mm, Logan:VIA-0.6mm, F.Cu at (106.2, 78.3)
- added REF**: VIA-0.6mm, Logan:VIA-0.6mm, F.Cu at (107.2, 78.3)
- added REF**: VIA-0.6mm, Logan:VIA-0.6mm, F.Cu at (108.2, 78.3)
- added REF**: VIA-0.6mm, Logan:VIA-0.6mm, F.Cu at (109.2, 78.3)
- added REF**: VIA-0.6mm, Logan:VIA-0.6mm, F.Cu at (110.2, 78.3)
- added REF**: VIA-0.6mm, Logan:VIA-0.6mm, F.Cu at (74.8, 82.5)
- added REF**: VIA-0.6mm, Logan:VIA-0.6mm, F.Cu at (92.4, 42.3)
- added REF**: VIA-0.6mm, Logan:VIA-0.6mm, F.Cu at (111.2, 78.3)
- added REF**: VIA-0.6mm, Logan:VIA-0.6mm, F.Cu at (112.2, 78.3)
- added REF**: VIA-0.6mm, Logan:VIA-0.6mm, F.Cu at (102.2, 78.3)
- added REF**: VIA-0.6mm, Logan:VIA-0.6mm, F.Cu at (103.2, 78.3)
- added REF**: VIA-0.6mm, Logan:VIA-0.6mm, F.Cu at (104.2, 77.3)
- added REF**: VIA-0.6mm, Logan:VIA-0.6mm, F.Cu at (105.2, 77.3)
- added REF**: VIA-0.6mm, Logan:VIA-0.6mm, F.Cu at (106.2, 77.3)
- added REF**: VIA-0.6mm, Logan:VIA-0.6mm, F.Cu at (107.2, 77.3)
- added REF**: VIA-0.6mm, Logan:VIA-0.6mm, F.Cu at (108.2, 77.3)
- added REF**: VIA-0.6mm, Logan:VIA-0.6mm, F.Cu at (109.2, 77.3)
- added REF**: VIA-0.6mm, Logan:VIA-0.6mm, F.Cu at (91.4, 42.3)
- added REF**: VIA-0.6mm, Logan:VIA-0.6mm, F.Cu at (110.2, 77.3)
- added REF**: VIA-0.6mm, Logan:VIA-0.6mm, F.Cu at (111.2, 77.3)
- added REF**: VIA-0.6mm, Logan:VIA-0.6mm, F.Cu at (112.2, 77.3)
- added REF**: VIA-0.6mm, Logan:VIA-0.6mm, F.Cu at (102.2, 77.3)
- added REF**: VIA-0.6mm, Logan:VIA-0.6mm, F.Cu at (103.2, 77.3)
- added REF**: VIA-0.6mm, Logan:VIA-0.6mm, F.Cu at (104.2, 76.3)
- added REF**: VIA-0.6mm, Logan:VIA-0.6mm, F.Cu at (105.2, 76.3)
- added REF**: VIA-0.6mm, Logan:VIA-0.6mm, F.Cu at (106.2, 76.3)
- added REF**: VIA-0.6mm, Logan:VIA-0.6mm, F.Cu at (107.2, 76.3)
- added REF**: VIA-0.6mm, Logan:VIA-0.6mm, F.Cu at (108.2, 76.3)
- added REF**: VIA-0.6mm, Logan:VIA-0.6mm, F.Cu at (90.4, 42.3)
- added REF**: VIA-0.6mm, Logan:VIA-0.6mm, F.Cu at (109.2, 76.3)
- added REF**: VIA-0.6mm, Logan:VIA-0.6mm, F.Cu at (110.2, 76.3)
- added REF**: VIA-0.6mm, Logan:VIA-0.6mm, F.Cu at (111.2, 76.3)
- added REF**: VIA-0.6mm, Logan:VIA-0.6mm, F.Cu at (112.2, 76.3)
- added REF**: VIA-0.6mm, Logan:VIA-0.6mm, F.Cu at (84.7, 78.3)
- added REF**: VIA-0.6mm, Logan:VIA-0.6mm, F.Cu at (85.7, 78.3)
- added REF**: VIA-0.6mm, Logan:VIA-0.6mm, F.Cu at (86.7, 78.3)
- added REF**: VIA-0.6mm, Logan:VIA-0.6mm, F.Cu at (87.7, 78.3)
- added REF**: VIA-0.6mm, Logan:VIA-0.6mm, F.Cu at (88.7, 78.3)
- added REF**: VIA-0.6mm, Logan:VIA-0.6mm, F.Cu at (89.7, 78.3)
- added REF**: VIA-0.6mm, Logan:VIA-0.6mm, F.Cu at (89.4, 42.3)
- added REF**: VIA-0.6mm, Logan:VIA-0.6mm, F.Cu at (90.7, 78.3)
- added REF**: VIA-0.6mm, Logan:VIA-0.6mm, F.Cu at (91.7, 78.3)
- added REF**: VIA-0.6mm, Logan:VIA-0.6mm, F.Cu at (92.7, 78.3)
- added REF**: VIA-0.6mm, Logan:VIA-0.6mm, F.Cu at (93.7, 78.3)
- added REF**: VIA-0.6mm, Logan:VIA-0.6mm, F.Cu at (94.7, 78.3)
- added REF**: VIA-0.6mm, Logan:VIA-0.6mm, F.Cu at (95.7, 78.3)
- added REF**: VIA-0.6mm, Logan:VIA-0.6mm, F.Cu at (96.7, 78.3)
- added REF**: VIA-0.6mm, Logan:VIA-0.6mm, F.Cu at (102.2, 76.3)
- added REF**: VIA-0.6mm, Logan:VIA-0.6mm, F.Cu at (103.2, 76.3)
- added REF**: VIA-0.6mm, Logan:VIA-0.6mm, F.Cu at (104.2, 75.3)
- added REF**: VIA-0.6mm, Logan:VIA-0.6mm, F.Cu at (88.4, 42.3)
- added REF**: VIA-0.6mm, Logan:VIA-0.6mm, F.Cu at (105.2, 75.3)
- added REF**: VIA-0.6mm, Logan:VIA-0.6mm, F.Cu at (106.2, 75.3)
- added REF**: VIA-0.6mm, Logan:VIA-0.6mm, F.Cu at (107.2, 75.3)
- added REF**: VIA-0.6mm, Logan:VIA-0.6mm, F.Cu at (108.2, 75.3)
- added REF**: VIA-0.6mm, Logan:VIA-0.6mm, F.Cu at (109.2, 75.3)
- added REF**: VIA-0.6mm, Logan:VIA-0.6mm, F.Cu at (110.2, 75.3)
- added REF**: VIA-0.6mm, Logan:VIA-0.6mm, F.Cu at (111.2, 75.3)
- added REF**: VIA-0.6mm, Logan:VIA-0.6mm, F.Cu at (112.2, 75.3)
- added REF**: VIA-0.6mm, Logan:VIA-0.6mm, F.Cu at (84.7, 77.3)
- added REF**: VIA-0.6mm, Logan:VIA-0.6mm, F.Cu at (85.7, 77.3)
- added REF**: VIA-0.6mm, Logan:VIA-0.6mm, F.Cu at (87.4, 42.3)
- added REF**: VIA-0.6mm, Logan:VIA-0.6mm, F.Cu at (86.7, 77.3)
- added REF**: VIA-0.6mm, Logan:VIA-0.6mm, F.Cu at (87.7, 77.3)
- added REF**: VIA-0.6mm, Logan:VIA-0.6mm, F.Cu at (88.7, 77.3)
- added REF**: VIA-0.6mm, Logan:VIA-0.6mm, F.Cu at (89.7, 77.3)
- added REF**: VIA-0.6mm, Logan:VIA-0.6mm, F.Cu at (90.7, 77.3)
- added REF**: VIA-0.6mm, Logan:VIA-0.6mm, F.Cu at (91.7, 77.3)
- added REF**: VIA-0.6mm, Logan:VIA-0.6mm, F.Cu at (92.7, 77.3)
- added REF**: VIA-0.6mm, Logan:VIA-0.6mm, F.Cu at (93.7, 77.3)
- added REF**: VIA-0.6mm, Logan:VIA-0.6mm, F.Cu at (94.7, 77.3)
- added REF**: VIA-0.6mm, Logan:VIA-0.6mm, F.Cu at (95.7, 77.3)
- added REF**: VIA-0.6mm, Logan:VIA-0.6mm, F.Cu at (86.4, 42.3)
- added REF**: VIA-0.6mm, Logan:VIA-0.6mm, F.Cu at (96.7, 77.3)
- added REF**: VIA-0.6mm, Logan:VIA-0.6mm, F.Cu at (102.2, 75.3)
- added REF**: VIA-0.6mm, Logan:VIA-0.6mm, F.Cu at (103.2, 75.3)
- added REF**: VIA-0.6mm, Logan:VIA-0.6mm, F.Cu at (104.2, 74.3)
- added REF**: VIA-0.6mm, Logan:VIA-0.6mm, F.Cu at (105.2, 74.3)
- added REF**: VIA-0.6mm, Logan:VIA-0.6mm, F.Cu at (106.2, 74.3)
- added REF**: VIA-0.6mm, Logan:VIA-0.6mm, F.Cu at (107.2, 74.3)
- added REF**: VIA-0.6mm, Logan:VIA-0.6mm, F.Cu at (108.2, 74.3)
- added REF**: VIA-0.6mm, Logan:VIA-0.6mm, F.Cu at (109.2, 74.3)
- added REF**: VIA-0.6mm, Logan:VIA-0.6mm, F.Cu at (110.2, 74.3)
- added REF**: VIA-0.6mm, Logan:VIA-0.6mm, F.Cu at (115.4, 43.3)
- added REF**: VIA-0.6mm, Logan:VIA-0.6mm, F.Cu at (111.2, 74.3)
- added REF**: VIA-0.6mm, Logan:VIA-0.6mm, F.Cu at (112.2, 74.3)
- added REF**: VIA-0.6mm, Logan:VIA-0.6mm, F.Cu at (84.7, 76.3)
- added REF**: VIA-0.6mm, Logan:VIA-0.6mm, F.Cu at (85.7, 76.3)
- added REF**: VIA-0.6mm, Logan:VIA-0.6mm, F.Cu at (86.7, 76.3)
- added REF**: VIA-0.6mm, Logan:VIA-0.6mm, F.Cu at (87.7, 76.3)
- added REF**: VIA-0.6mm, Logan:VIA-0.6mm, F.Cu at (88.7, 76.3)
- added REF**: VIA-0.6mm, Logan:VIA-0.6mm, F.Cu at (89.7, 76.3)
- added REF**: VIA-0.6mm, Logan:VIA-0.6mm, F.Cu at (90.7, 76.3)
- added REF**: VIA-0.6mm, Logan:VIA-0.6mm, F.Cu at (91.7, 76.3)
- added REF**: VIA-0.6mm, Logan:VIA-0.6mm, F.Cu at (114.4, 43.3)
- added REF**: VIA-0.6mm, Logan:VIA-0.6mm, F.Cu at (92.7, 76.3)
- added REF**: VIA-0.6mm, Logan:VIA-0.6mm, F.Cu at (93.7, 76.3)
- added REF**: VIA-0.6mm, Logan:VIA-0.6mm, F.Cu at (94.7, 76.3)
- added REF**: VIA-0.6mm, Logan:VIA-0.6mm, F.Cu at (95.7, 76.3)
- added REF**: VIA-0.6mm, Logan:VIA-0.6mm, F.Cu at (96.7, 76.3)
- added REF**: VIA-0.6mm, Logan:VIA-0.6mm, F.Cu at (102.2, 74.3)
- added REF**: VIA-0.6mm, Logan:VIA-0.6mm, F.Cu at (103.2, 74.3)
- added REF**: VIA-0.6mm, Logan:VIA-0.6mm, F.Cu at (57.2, 103.7)
- added REF**: VIA-0.6mm, Logan:VIA-0.6mm, F.Cu at (58.2, 103.7)
- added REF**: VIA-0.6mm, Logan:VIA-0.6mm, F.Cu at (59.2, 103.7)
- added REF**: VIA-0.6mm, Logan:VIA-0.6mm, F.Cu at (113.4, 43.3)
- added REF**: VIA-0.6mm, Logan:VIA-0.6mm, F.Cu at (60.2, 103.7)
- added REF**: VIA-0.6mm, Logan:VIA-0.6mm, F.Cu at (61.2, 103.7)
- added REF**: VIA-0.6mm, Logan:VIA-0.6mm, F.Cu at (62.2, 103.7)
- added REF**: VIA-0.6mm, Logan:VIA-0.6mm, F.Cu at (63.2, 103.7)
- added REF**: VIA-0.6mm, Logan:VIA-0.6mm, F.Cu at (64.2, 103.7)
- added REF**: VIA-0.6mm, Logan:VIA-0.6mm, F.Cu at (65.2, 103.7)
- added REF**: VIA-0.6mm, Logan:VIA-0.6mm, F.Cu at (66.2, 103.7)
- added REF**: VIA-0.6mm, Logan:VIA-0.6mm, F.Cu at (67.2, 103.7)
- added REF**: VIA-0.6mm, Logan:VIA-0.6mm, F.Cu at (68.2, 103.7)
- added REF**: VIA-0.6mm, Logan:VIA-0.6mm, F.Cu at (69.2, 103.7)
- added REF**: VIA-0.6mm, Logan:VIA-0.6mm, F.Cu at (74.8, 83.5)
- added REF**: VIA-0.6mm, Logan:VIA-0.6mm, F.Cu at (112.4, 43.3)
- added REF**: VIA-0.6mm, Logan:VIA-0.6mm, F.Cu at (70.2, 103.7)
- added REF**: VIA-0.6mm, Logan:VIA-0.6mm, F.Cu at (71.2, 103.7)
- added REF**: VIA-0.6mm, Logan:VIA-0.6mm, F.Cu at (72.2, 103.7)
- added REF**: VIA-0.6mm, Logan:VIA-0.6mm, F.Cu at (73.2, 103.7)
- added REF**: VIA-0.6mm, Logan:VIA-0.6mm, F.Cu at (74.2, 103.7)
- added REF**: VIA-0.6mm, Logan:VIA-0.6mm, F.Cu at (75.2, 103.7)
- added REF**: VIA-0.6mm, Logan:VIA-0.6mm, F.Cu at (59.2, 102.7)
- added REF**: VIA-0.6mm, Logan:VIA-0.6mm, F.Cu at (60.2, 102.7)
- added REF**: VIA-0.6mm, Logan:VIA-0.6mm, F.Cu at (61.2, 102.7)
- added REF**: VIA-0.6mm, Logan:VIA-0.6mm, F.Cu at (62.2, 102.7)
- added REF**: VIA-0.6mm, Logan:VIA-0.6mm, F.Cu at (111.4, 43.3)
- added REF**: VIA-0.6mm, Logan:VIA-0.6mm, F.Cu at (63.2, 102.7)
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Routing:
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- added copper zone on 5V0, net /DC Driver/OUT+
- added copper zone on B.Cu, net /DC Driver/OUT+
- added copper zone on GND, net /DC Driver/OUT+
- added copper zone on 5V0, net GND
- added copper zone on B.Cu, net GND
- added copper zone on F.Cu, net Net-(Q1-Pad1)
- added copper zone on 5V0, net Net-(Q1-Pad2)
- added copper zone on B.Cu, net Net-(Q1-Pad2)
- added copper zone on GND, net Net-(Q1-Pad2)
